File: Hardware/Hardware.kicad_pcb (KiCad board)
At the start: 2 copper layers, 102.9 x 121.9 mm, 39 parts, among them J2 RJ45_LED_Shielded, J3 USB_A, J5 Conn_01x06_Pin, SW1 SW_SPST, SW14 SW_Push, SW2 SW_Push, SW3 SW_Push, SW4 SW_Push, SW5 SW_Push, SW6 SW_Push, SW7 SW_Push, U1 TMR-0511, U2 ATA6561, U3 Teensy4.1_DEV-16771, U4 ESP32-WROOM-32UE, U5 ASSR-1218, U6 ASSR-1218

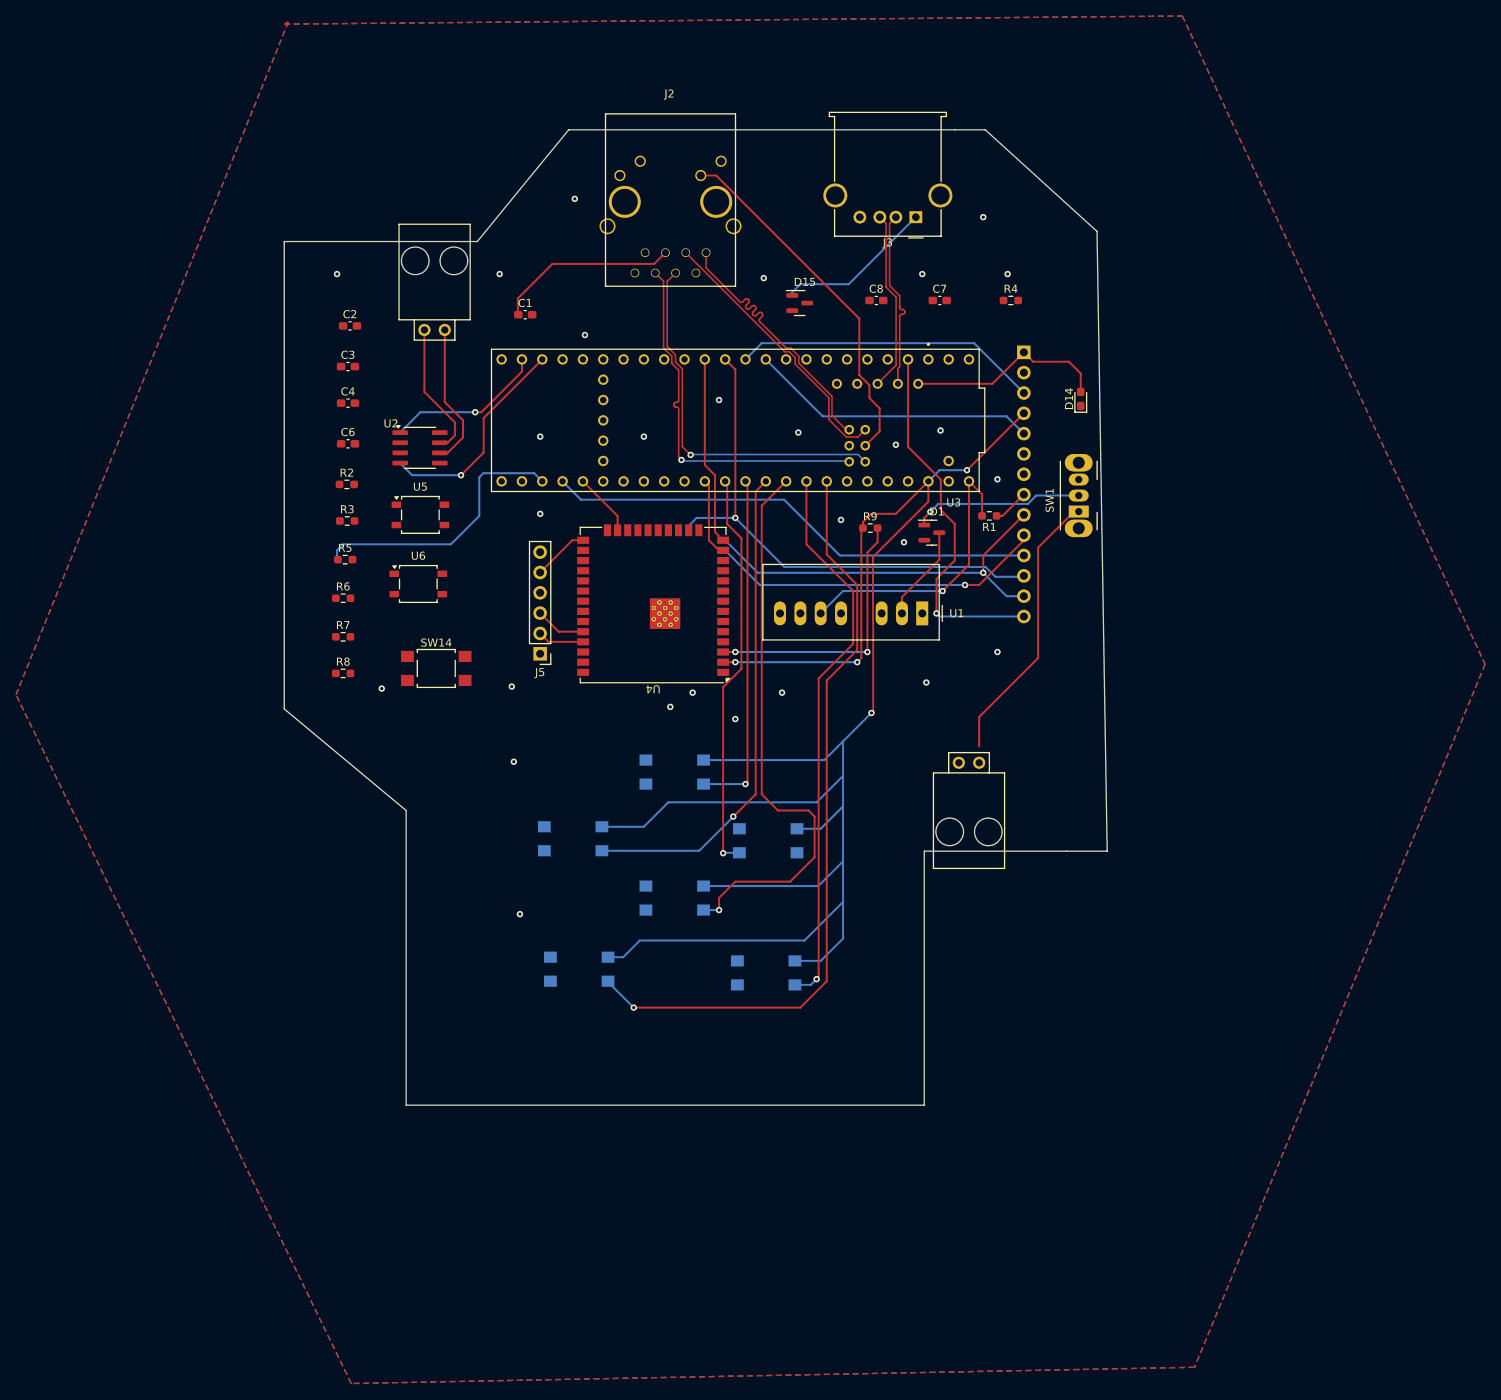
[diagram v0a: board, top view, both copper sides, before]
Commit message: finished up the layout and cleaned up libraries
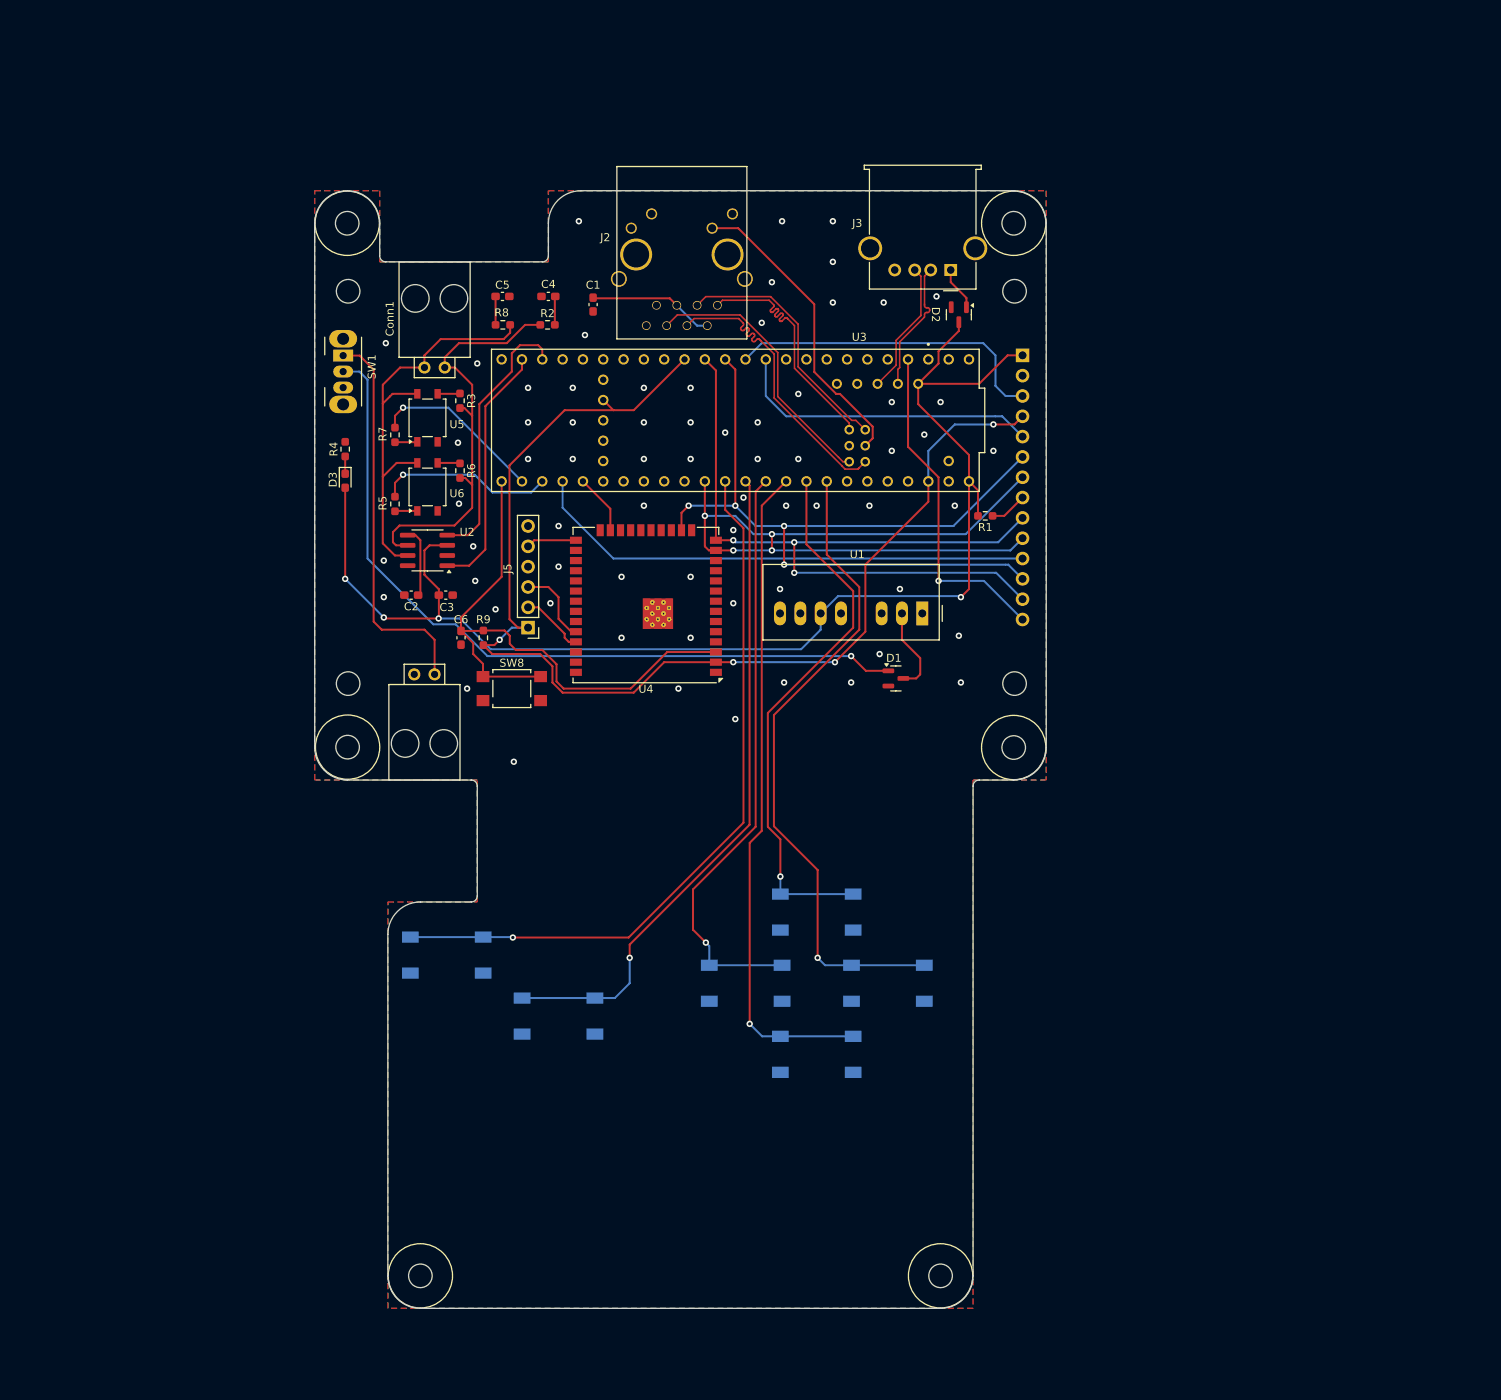
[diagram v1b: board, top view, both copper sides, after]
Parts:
- removed C7: 0.1uF, Capacitor_SMD:C_0603_1608Metric_Pad1.08x0.95mm_HandSolder
- removed C8: 1uF, Capacitor_SMD:C_0603_1608Metric_Pad1.08x0.95mm_HandSolder
- added C5: 4.7nF, Capacitor_SMD:C_0603_1608Metric_Pad1.08x0.95mm_HandSolder, F.Cu at (177.1, 74.2)
- added H1: MountingHole, MRDT_Drill_Holes:4_40_Hole, F.Cu at (241.0, 65.0)
- added H2: MountingHole, MRDT_Drill_Holes:4_40_Hole, F.Cu at (157.7, 65.0)
- added H3: MountingHole, MRDT_Drill_Holes:4_40_Hole, F.Cu at (241.0, 130.6)
- added H4: MountingHole, MRDT_Drill_Holes:4_40_Hole, F.Cu at (157.8, 130.5)
- added H5: MountingHole, MRDT_Drill_Holes:4_40_Hole, F.Cu at (166.9, 196.6)
- added H6: MountingHole, MRDT_Drill_Holes:4_40_Hole, F.Cu at (231.9, 196.6)
- C6: value 4.7nF -> 1uF
- D1: value D_Schottky -> D_Schottky_ZLLS500; footprint MRDT_Passives:SOT-23_Diode -> Tester:D_Schottky_ZLLS500
- D2: renamed from D15; value D_Schottky -> D_Schottky_ZLLS500; footprint MRDT_Passives:SOT-23_Diode -> Tester:D_Schottky_ZLLS500
- SW2, SW3, SW4, SW5, SW6, SW7: footprint Button_Switch_SMD:SW_SPST_TL3305A -> Tester:SW_SPST_TL3301
- U7: footprint sw_spst:DISPLAY_ILI9341_TOUCH_32 -> Tester:DISPLAY_ILI9341_TOUCH_32
- moved SW1 94.0 mm to (157.2, 81.6), turned to -90 degrees
- moved D3 92.5 mm to (157.5, 97.2), turned to -90 degrees
- moved R4 85.3 mm to (157.5, 93.3), turned to 90 degrees
- moved BT1 69.0 mm to (168.7, 121.4)
- moved R9 50.3 mm to (174.8, 116.8), turned to 90 degrees
- moved R8 47.9 mm to (177.2, 77.7), turned to 180 degrees
- moved SW2 42.6 mm to (170.2, 156.5), turned to 0 degrees
- moved SW7 38.6 mm to (225.3, 160.0), turned to 0 degrees
- moved C2 34.5 mm to (165.7, 111.5), turned to 180 degrees
- moved SW3 33.8 mm to (184.2, 164.1), turned to 0 degrees
- moved R2 32.1 mm to (182.8, 77.7)
- moved C3 31.1 mm to (170.1, 111.5)
- moved C4 28.4 mm to (182.9, 74.2), turned to 180 degrees
- moved SW4 28.1 mm to (207.5, 160.0), turned to 0 degrees
- moved C6 28.1 mm to (172.0, 116.8), turned to -90 degrees
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- renumbered D14 to D3, SW14 to SW8
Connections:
- net kp_button1 renamed KP_ACCEPT
- net kp_button2 renamed KP_BACK
- net kp_button3 renamed KP_RIGHT
- net kp_button6 renamed KP_LEFT
- C6 pad 1: Net-(C6-Pad1) -> WiFi_EN
- D1 pad 2: Net-(D1-A) -> unconnected-(D1-NC-Pad2)
- D1 pad 3: (no net) -> Net-(D1-A)
- D2 pad 2: Net-(D15-A) -> unconnected-(D2-NC-Pad2)
- D2 pad 3: (no net) -> Net-(D2-A)
- J3 pad 1: Net-(D15-A) -> Net-(D2-A)
- R8 pad 2: Net-(C6-Pad1) -> Net-(C5-Pad1)
- SW2 pad 1: +3V3 -> GND
- SW3 pad 1: +3V3 -> GND
- SW4 pad 1: +3V3 -> GND
- SW5 pad 1: +3V3 -> GND
- SW5 pad 2: kp_button4 -> KP_UP
- SW6 pad 1: +3V3 -> GND
- SW6 pad 2: kp_button5 -> KP_DOWN
- SW7 pad 1: +3V3 -> GND
- U3 pad 17: kp_button4 -> KP_DOWN
- U3 pad 18: kp_button5 -> KP_UP
- U3 pad 33: unconnected-(U3-MCLK2-Pad33) -> WiFi_EN
- U3 pad D-: (no net) -> USB_D-
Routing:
- net +5V: track 62.1 -> 167.5 mm, vias 1 -> 4
- net +3V3: track 238.6 -> 151.2 mm
- net KP_DOWN: track 0.00 -> 83.3 mm, vias 0 -> 1
- net Net-(D1-A): track 21.4 -> 96.8 mm
- net kp_button4: track 70.7 -> 0.00 mm, vias 1 -> 0
- net kp_button5: track 69.5 -> 0.00 mm, vias 1 -> 0
- net KP_UP: track 0.00 -> 68.2 mm, vias 0 -> 1
- net SCK: track 51.8 -> 94.6 mm, vias 1 -> 4
- net KP_ACCEPT: track 50.3 -> 91.2 mm
- net KP_BACK: track 43.9 -> 83.6 mm
- net WiFi_EN: track 34.1 -> 73.5 mm, vias 2 -> 0
- net MOSI: track 66.1 -> 104.3 mm, vias 1 -> 4
- net Net-(U2-CANH): track 17.0 -> 53.9 mm
- net Net-(U2-CANL): track 18.1 -> 52.8 mm
- net MISO: track 73.1 -> 96.9 mm, vias 1 -> 3
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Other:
- board size 102.9 x 121.9 mm -> 91.4 x 139.7 mm
- board text added: "Accept"
- board text added: "Back"
